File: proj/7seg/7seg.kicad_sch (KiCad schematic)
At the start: 40 parts, among them J1 Conn_01x03_Pin, J3 UART, J4 UART, J9 USB_C, U1 74HC595, U10 D168K, U11 MCU_DISP, U12 MCU_CTL, U13 CH340E, U14 CH340K, U2 74HC595, U3 D168K, U4 D168K, U5 D168K, U6 D168K, U7 D168K, U8 D168K, U9 D168K

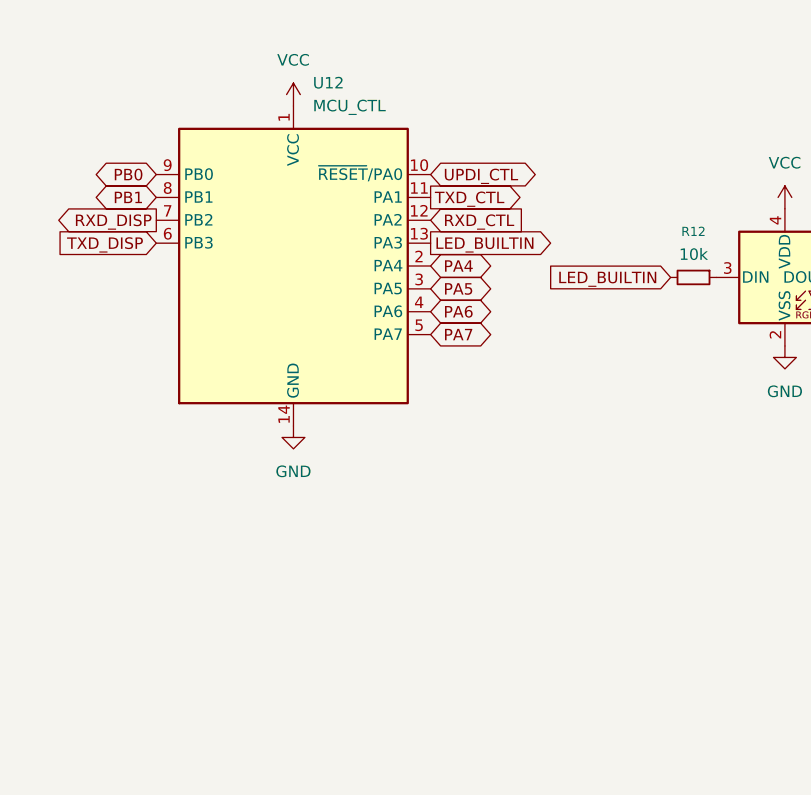
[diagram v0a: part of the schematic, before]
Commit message: -
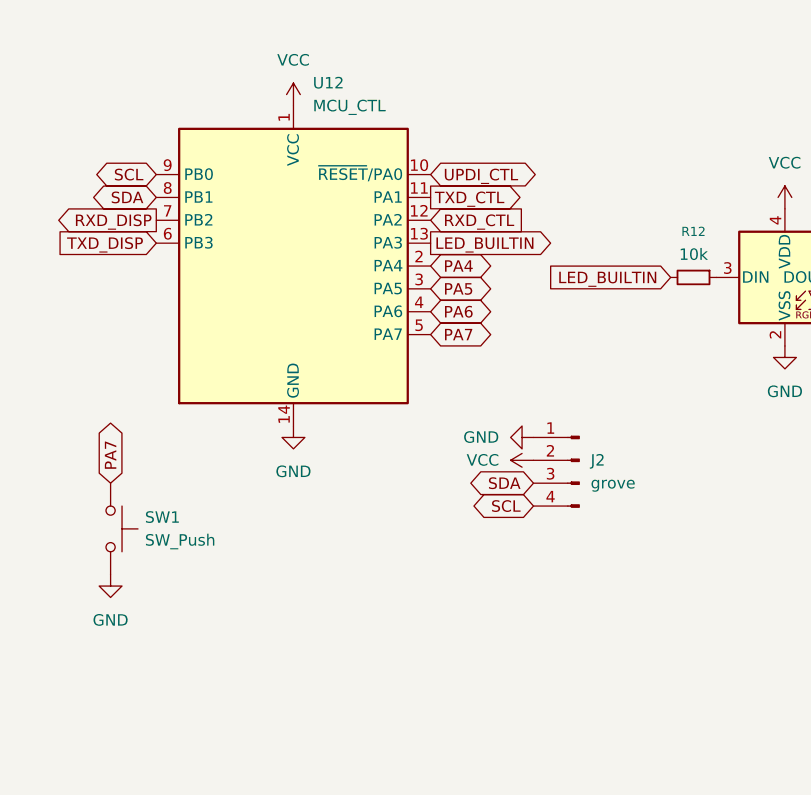
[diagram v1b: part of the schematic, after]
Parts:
- added J2: grove, Connector_PinHeader_2.54mm:PinHeader_1x04_P2.54mm_Vertical, symbol Connector:Conn_01x04_Pin
- added SW1: SW_Push, Library:alps-skrp, symbol Switch:SW_Push
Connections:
- net GND: now also J2.1 (Pin_1), SW1.2
- net PA7: now also SW1.1
- net VCC: now also J2.2 (Pin_2)
- net PB0 renamed SCL
- net SCL: now also J2.4 (Pin_4)
- net PB1 renamed SDA
- net SDA: now also J2.3 (Pin_3)
